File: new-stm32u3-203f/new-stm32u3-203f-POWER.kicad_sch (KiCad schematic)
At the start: 31 parts, among them J4 Battery connector, SW2 SW_SPDT, U4 LD39050PU33R, U5 TLV62569DBVR, U6 MCP73831T-2ACI/OT, U7 TPS63802DLAR

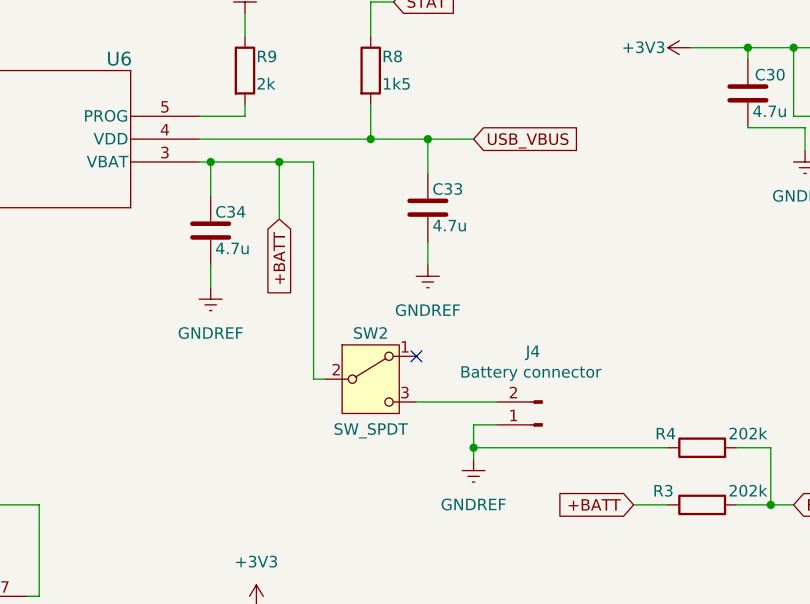
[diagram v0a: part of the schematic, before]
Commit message: finished the layout of the pcb
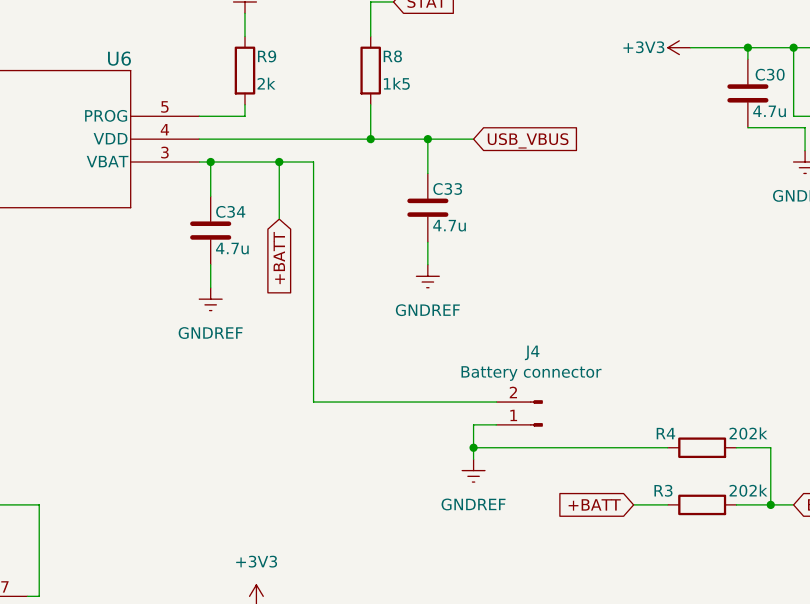
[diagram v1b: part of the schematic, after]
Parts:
- removed SW2: SW_SPDT, footprints_SPDT_slide:CL-SB-12B-01_NDC, symbol Switch:SW_SPDT
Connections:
- net +BATT: now also J4.2 (Pin_2)
- no-connect marks 2 -> 1
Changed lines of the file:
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@@
 		(at 171.45 41.91)
 	)
-	(no_connect
-		(at 127 105.41)
-	)
 	(wire
 		(pts
@@
 	(wire
 		(pts
-			(xy 127 110.49) (xy 135.89 110.49)
-		)
-		(stroke
-			(width 0)
-			(type default)
-		)
-	)
-	(wire
-		(pts
 			(xy 166.37 115.57) (xy 162.56 115.57)
 		)
@@
 	(wire
 		(pts
-			(xy 115.57 107.95) (xy 115.57 83.82)
+			(xy 115.57 110.49) (xy 115.57 83.82)
 		)
 		(stroke
@@
 	(wire
 		(pts
-			(xy 115.57 107.95) (xy 116.84 107.95)
+			(xy 115.57 110.49) (xy 135.89 110.49)
 		)
 		(stroke
@@
 					(unit 1)
 				)
-			)
-		)
-	)
-	(symbol
-		(lib_id "Switch:SW_SPDT")
-		(at 121.92 107.95 0)
-		(unit 1)
-		(exclude_from_sim no)
-		(in_bom yes)
-		(on_board yes)
-		(dnp no)
-		(property "Reference" "SW2"
-			(at 121.92 102.87 0)
-			(effects
-				(font
-					(size 1.27 1.27)
-				)
-			)
-		)
-		(property "Value" "SW_SPDT"
-			(at 121.92 113.538 0)
-			(effects
-				(font
-					(size 1.27 1.27)
-				)
-			)
-		)
-		(property "Footprint" "footprints_SPDT_slide:CL-SB-12B-01_NDC"
-			(at 121.92 107.95 0)
-			(effects
-				(font
-					(size 1.27 1.27)
-				)
-				(hide yes)
-			)
-		)
-		(property "Datasheet" "~"
-			(at 121.92 115.57 0)
-			(effects
-				(font
-					(size 1.27 1.27)
-				)
-				(hide yes)
-			)
-		)
-		(property "Description" "Switch, single pole double throw"
-			(at 121.92 107.95 0)
-			(effects
-				(font
-					(size 1.27 1.27)
-				)
-				(hide yes)
-			)
-		)
-		(pin "1"
-		)
-		(pin "3"
-		)
-		(pin "2"
-		)
-		(instances
-			(project ""
-				(path "/133609ce-1e1a-4c9a-bce3-37a0219dc965/fbdd0d38-3709-4a96-99fb-af9d998b7f91"
-					(reference "SW2")
-					(unit 1)
-				)
